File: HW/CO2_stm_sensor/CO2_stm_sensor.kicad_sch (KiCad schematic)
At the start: 41 parts, among them IC1 SCD41-D-R2, IC2 TPS22917DBVR, IC3 TPS22917DBVR, J1 DM3D-SF(41), J2 SWD, J3 LP_UART, J4 DBG_UART, J5 BATTERY, J6 10118193-0001LF, U1 STM32L021K4T6, U2 TPS7A0228PDBVR

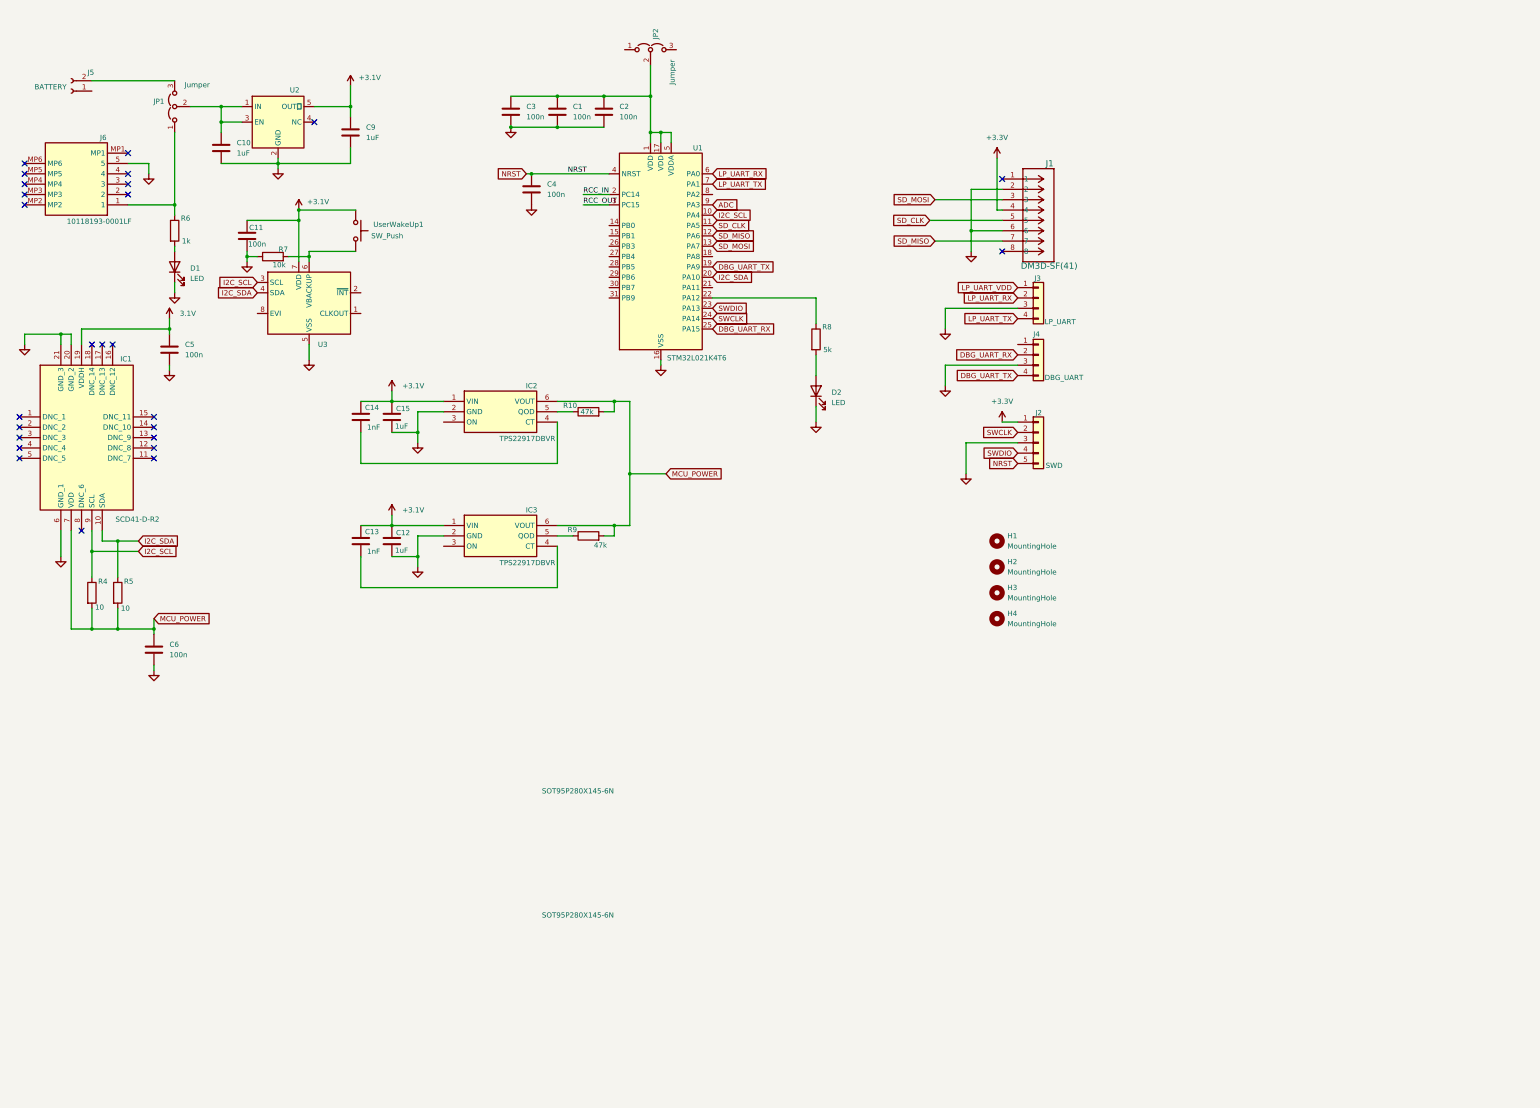
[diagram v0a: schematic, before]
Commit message: shchematic v0.0 done
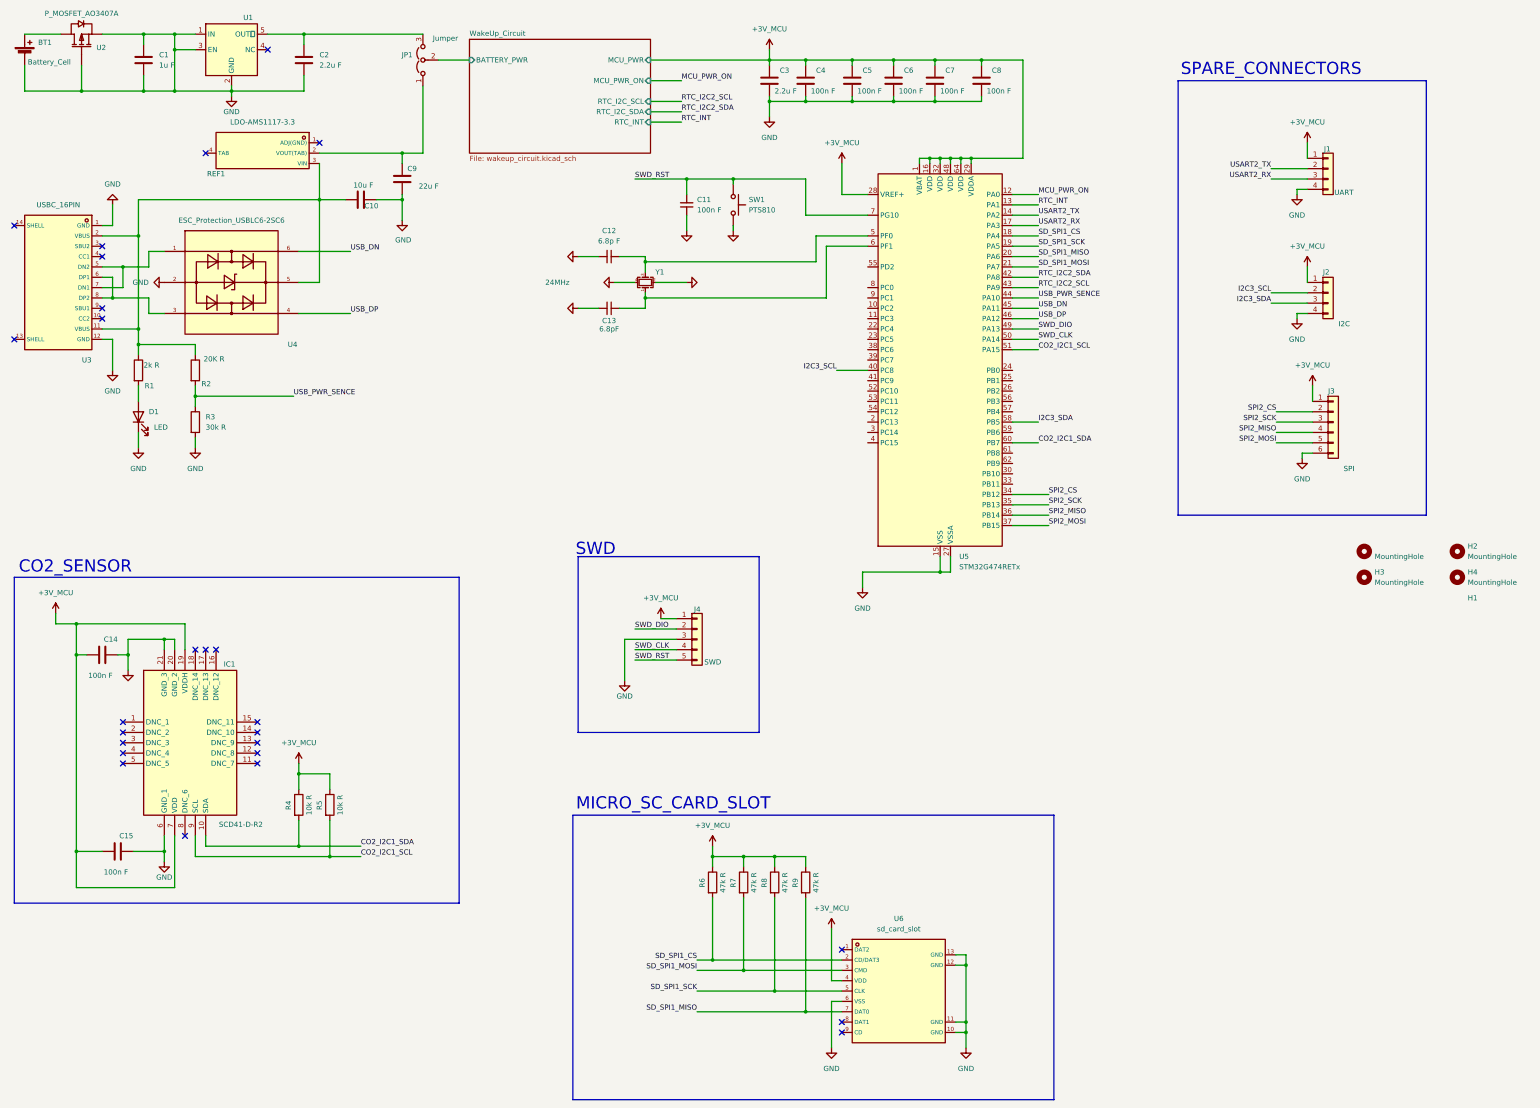
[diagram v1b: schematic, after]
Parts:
- removed C11, C2: 100n, symbol Device:C
- removed C12: 1uF, symbol Device:C
- removed C13: 1nF, symbol Device:C
- removed D2: LED, symbol Device:LED
- removed IC2, IC3: TPS22917DBVR, SOT95P280X145-6N, symbol TPS22917DBVR:TPS22917DBVR
- removed J1: DM3D-SF(41), CONN8_DM3D-SF_HIR, symbol sd_card:DM3D-SF
- removed J5: BATTERY, symbol Connector:Conn_01x02_Socket
- removed J6: 10118193-0001LF, 101181920002LF, symbol 10118192-0002LF:10118192-0002LF
- removed JP2: Jumper, symbol Jumper:Jumper_3_Open
- removed R10: 47k, symbol Device:R
- removed U1: STM32L021K4T6, Package_QFP:LQFP-32_7x7mm_P0.8mm, symbol MCU_ST_STM32L0:STM32L021K4Tx
- removed U3: ~, Package_SON:MicroCrystal_C7_SON-8_1.5x3.2mm_P0.9mm, symbol Timer_RTC:RV-3028-C7
- removed UserWakeUp1: SW_Push, symbol Switch:SW_Push
- added BT1: Battery_Cell, symbol Device:Battery_Cell
- added C11: 100n F, Capacitor_SMD:C_0805_2012Metric_Pad1.18x1.45mm_HandSolder, symbol Device:C_Small
- added C12: 6.8p F, Capacitor_SMD:C_0805_2012Metric_Pad1.18x1.45mm_HandSolder, symbol Device:C_Small
- added C13: 6.8pF, Capacitor_SMD:C_0805_2012Metric_Pad1.18x1.45mm_HandSolder, symbol Device:C_Small
- added C7, C8: 100n F, symbol Device:C
- added C9: 22u F, symbol Device:C
- added J3: SPI, symbol Connector_Generic:Conn_01x06
- added R2: 20K R, symbol Device:R
- added R3: 30k R, symbol Device:R
- added R6: 47k R, symbol Device:R
- added REF1: LDO-AMS1117-3.3, JLC:SOT-223-4_L6.5-W3.5-P2.30-LS7.0-BR, symbol JLC:LDO-AMS1117-3.3
- added SW1: PTS810, Button_Switch_SMD:SW_SPST_PTS810, symbol teser_lib:button
- added U2: P_MOSFET_AO3407A, JLC:SOT-23-3_L2.9-W1.6-P1.90-LS2.8-BR, symbol JLC:P_MOSFET_AO3407A
- added U3: USBC_16PIN, JLC:USB-C-SMD_TYPE-C-6PIN-2MD-073, symbol JLC:USBC_16PIN
- added U4: ESC_Protection_USBLC6-2SC6, JLC:SOT-23-6_L2.9-W1.6-P0.95-LS2.8-BL, symbol JLC:ESC_Protection_USBLC6-2SC6
- added U5: STM32G474RETx, Package_QFP:LQFP-64_10x10mm_P0.5mm, symbol MCU_ST_STM32G4:STM32G474RETx
- added U6: sd_card_slot, JLC:TF-SMD_TF-CARD-H1.8, symbol JLC:sd_card_slot
- added Y1: 24MHz, teser_lib:crystal-24MHz, symbol Device:Crystal_GND24_Small
- C1: value 100n -> 1u F
- C10: value 1uF -> 10u F
- C14: value 1nF -> 100n F
- C15: value 1uF -> 100n F
- C2: renamed from C9; value 1uF -> 2.2u F
- C3: value 100n -> 2.2u F
- C4, C5, C6: value 100n -> 100n F
- J1: renamed from J3; value LP_UART -> UART
- J2: renamed from J4; value DBG_UART -> I2C
- R1: renamed from R6; value 1k -> 2k R
- R4, R5: value 10 -> 10k R
- R7: value 10k -> 47k R
- R8: value 5k -> 47k R
- R9: value 47k -> 47k R
- renumbered H3 to H1, H1 to H2, H4 to H3, H2 to H4, J2 to J4, U2 to U1
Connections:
- net +3.3V is gone; now on net +3V_MCU: J4.1 (Pin_1)
- net 3.1V is gone; now on net +3V_MCU: C5.1, IC1.19 (VDDH)
- net DBG_UART_TX is gone; now on net GND: J2.4 (Pin_4)
- net LP_UART_TX is gone; now on net GND: J1.4 (Pin_4)
- net LP_UART_VDD is gone; now on net +3V_MCU: J1.1 (Pin_1)
- net +3V_MCU: now reaches R7.1
- net +3V_MCU: now also C14.1, C15.1, C3.1, C4.1, C6.1, IC1.7 (VDD), J2.1 (Pin_1), R4.1, R5.1, R8.1, R9.1, C7.1, C8.1, J3.1 (Pin_1), R6.1, U5.1 (VBAT), U5.16 (VDD), U5.28 (VREF+), U5.29 (VDDA), U5.32 (VDD), U5.48 (VDD), U5.64 (VDD), U6.4 (VDD)
- net SD_SPI1_MOSI: now reaches R7.2
- net SD_SPI1_MOSI: now also U5.21 (PA7), U6.3 (CMD)
- net GND: now reaches C4.2
- net GND: now also C1.1, C1.2, C10.2, C14.2, C15.2, C2.2, C3.2, C5.2, C6.2, D1.1 (K), IC1.20 (GND_2), IC1.21 (GND_3), IC1.6 (GND_1), J4.3 (Pin_3), U1.1 (IN), U1.2 (GND), U1.3 (EN), BT1.2 (-), C11.1, C12.2, C13.2, C7.2, C8.2, C9.2, J3.6 (Pin_6), R3.2, SW1.2, U2.1 (G), U2.2 (S), U3.1 (GND), U3.12 (GND), U4.2, U5.15 (VSS), U5.27 (VSSA), U5.31 (VSS), U5.47 (VSS), U5.63 (VSS), U6.10 (GND), U6.11 (GND), U6.12 (GND), U6.13 (GND), U6.6 (VSS), Y1.2, Y1.4
- net at R1.1: now also C10.1, R2.1, REF1.3 (VIN), U3.11 (VBUS), U3.2 (VBUS), U4.5; no longer JP1.1 (A)
- net SD_SPI1_SCK: now reaches R8.2
- net SD_SPI1_SCK: now also U5.19 (PA5), U6.5 (CLK)
- net I2C3_SDA: now reaches J2.3 (Pin_3)
- net I2C3_SDA: now also U5.58 (PB5)
- net USART2_RX: now reaches J1.3 (Pin_3)
- net USART2_RX: now also U5.17 (PA3)
- net at JP1.3 (B): now also C2.1, U1.5 (OUT )
- removed net +3.1V: C14.1, C15.1, C2.1, U1.5 (OUT )
- net DBG_UART_RX renamed I2C3_SCL
- net I2C3_SCL: now also U5.40 (PC8)
- net I2C_SCL renamed CO2_I2C1_SCL
- net CO2_I2C1_SCL: now also R5.2, U5.51 (PA15); no longer R4.1
- net I2C_SDA renamed CO2_I2C1_SDA
- net CO2_I2C1_SDA: now also R4.2, U5.60 (PB7); no longer R5.1
- net LP_UART_RX renamed USART2_TX
- net USART2_TX: now also U5.14 (PA2)
- removed net MCU_POWER: C6.1, IC1.7 (VDD), R4.2, R5.2, R9.2
- net NRST renamed SWD_RST
- net SWD_RST: now also C11.2, SW1.1, U5.7 (PG10); no longer C4.1
- net SWCLK renamed SWD_DIO
- net SWD_DIO: now also U5.49 (PA13)
- net SWDIO renamed SWD_CLK
- net SWD_CLK: now also U5.50 (PA14)
- new net: C13.1, U5.6 (PF1), Y1.1
- new net: C9.1, JP1.1 (A), REF1.2 (VOUT(TAB))
- new net: BT1.1 (+), U2.3 (D)
- new net: C12.1, U5.5 (PF0), Y1.3
- new net: U3.5 (DN2), U3.7 (DN1), U4.1
- new net: U3.6 (DP1), U3.8 (DP2), U4.3
- new net MCU_PWR_ON: U5.12 (PA0)
- new net RTC_I2C2_SCL: U5.43 (PA9)
- new net RTC_I2C2_SDA: U5.42 (PA8)
- new net RTC_INT: U5.13 (PA1)
- new net SD_SPI1_CS: R6.2, U5.18 (PA4), U6.2 (CD/DAT3)
- new net SD_SPI1_MISO: R9.2, U5.20 (PA6), U6.7 (DAT0)
- new net SPI2_CS: J3.2 (Pin_2), U5.34 (PB12)
- new net SPI2_MISO: J3.4 (Pin_4), U5.36 (PB14)
- new net SPI2_MOSI: J3.5 (Pin_5), U5.37 (PB15)
- new net SPI2_SCK: J3.3 (Pin_3), U5.35 (PB13)
- new net USB_DN: U4.6, U5.45 (PA11)
- new net USB_DP: U4.4, U5.46 (PA12)
- new net USB_PWR_SENCE: R2.2, R3.1, U5.44 (PA10)
- new net WakeUp_Circuit/BATTERY_PWR: JP1.2 (C)
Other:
- added sheet WakeUp_Circuit (wakeup_circuit.kicad_sch)
- note added: "CO2_SENSOR"
- note added: "MICRO_SC_CARD_SLOT"
- note added: "SPARE_CONNECTORS"
- note added: "SWD"
- title: (none) -> CO2_stm32_sensor
- moved on the sheet: C2, D1, H1, H2, H3, H4, IC1, J1, J2, J4, JP1, R1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
